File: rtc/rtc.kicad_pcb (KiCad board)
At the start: 2 copper layers, 23.5 x 32.4 mm, 17 parts, among them J1 Conn_02x03_Odd_Even, J2 Conn_01x04, J3 Conn_01x04, J4 Conn_01x04, U1 PCF8563T/5_518, Y1 LFXTAL016178REEL

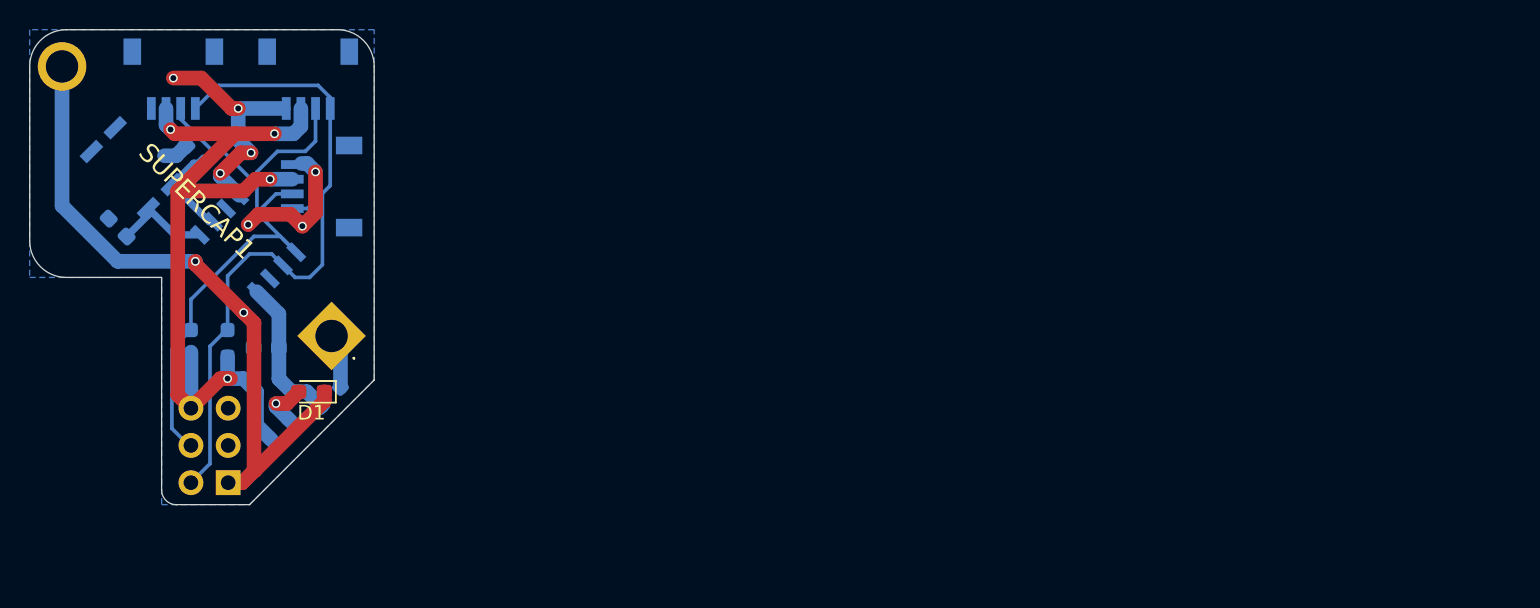
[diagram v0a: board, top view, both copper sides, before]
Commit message: rtc_commit
pushed to git properly
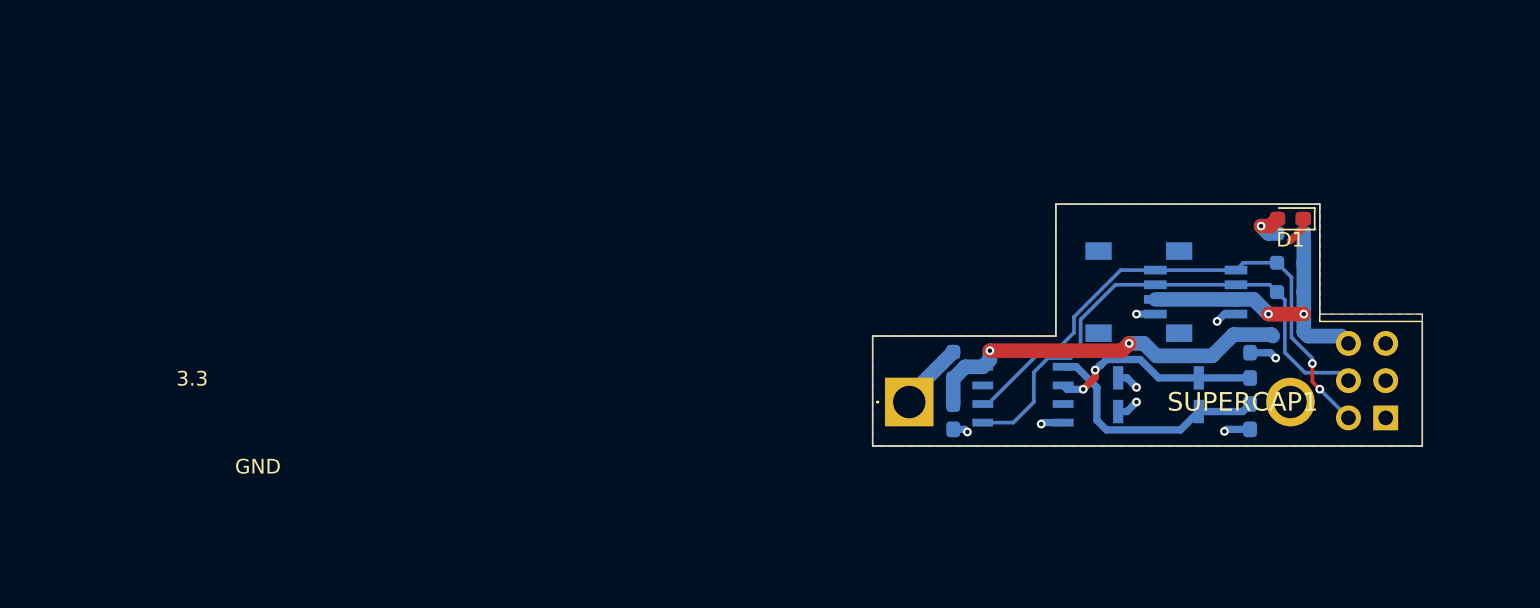
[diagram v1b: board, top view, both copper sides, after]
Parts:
- removed J4: Conn_01x04, pcb_footprints:SM04BSRSSTB
- moved J1 79.1 mm to (233.5, 94.1)
- moved C1 78.3 mm to (224.2, 94.0), turned to -90 degrees
- moved R2 75.1 mm to (227.0, 85.5), turned to 0 degrees
- moved C3 73.4 mm to (224.2, 90.5), turned to 90 degrees
- moved R3 72.7 mm to (227.0, 83.5), turned to 0 degrees
- moved Y1 71.7 mm to (218.0, 92.5), turned to 180 degrees
- moved G*** 70.8 mm to (214.0, 82.5), turned to 180 degrees
- moved R4 70.2 mm to (227.0, 81.5), turned to 180 degrees
- moved D2 69.4 mm to (227.0, 88.5), turned to 0 degrees
- moved D1 67.8 mm to (227.0, 80.5)
- moved J3 60.2 mm to (221.0, 85.5), turned to 90 degrees
- moved J2 57.4 mm to (215.5, 85.5), turned to 90 degrees
- moved U1 53.9 mm to (208.8, 92.5), turned to 180 degrees
- moved C2 47.1 mm to (204.0, 94.0), turned to -90 degrees
- moved R1 42.5 mm to (204.0, 90.5), turned to -90 degrees
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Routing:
- net GND: track 76.1 -> 14.0 mm, vias 9 -> 8
- net +3.3V: track 55.8 -> 20.1 mm, vias 4 -> 2
- net Net-(D2-K): track 10.3 -> 25.9 mm, vias 0 -> 2
- net scl: track 48.3 -> 37.5 mm, vias 0 -> 2
- net Net-(U1-OSCI): track 6.78 -> 16.6 mm
- net sda: track 45.3 -> 36.0 mm
- net Net-(U1-OSCO): track 6.47 -> 14.5 mm, vias 0 -> 2
- net Net-(SUPERCAP1-+): track 3.76 -> 4.66 mm
- net Net-(D1-A): track 3.43 -> 2.63 mm
- added copper zone on F.Cu, net GND
- removed copper zone on B.Cu, net GND
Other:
- board size 23.5 x 32.4 mm -> 37.5 x 16.5 mm
- board text added: "3.3"
- board text added: "GND"
- board text added: "Made by Hailin Chen"
- board text removed: "Designed by A. Ai"

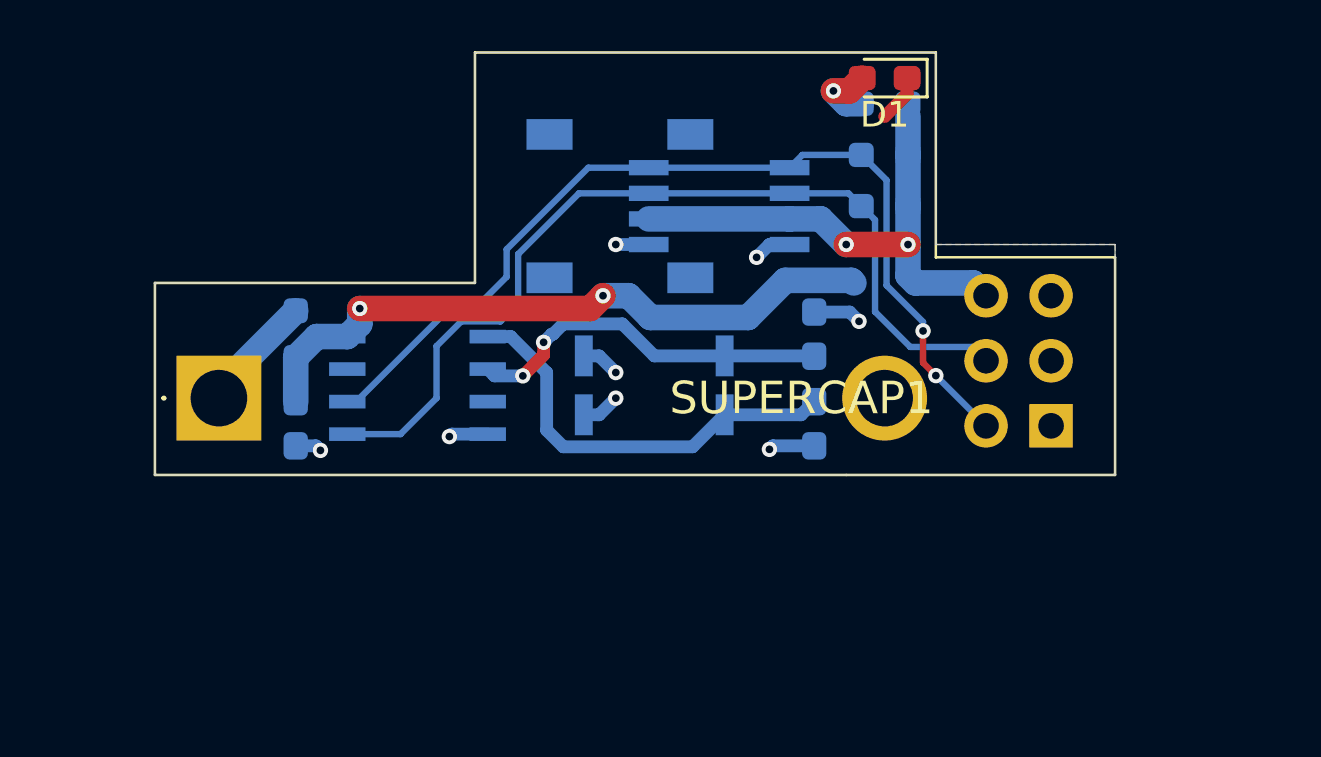
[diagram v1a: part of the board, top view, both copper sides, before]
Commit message: Update rtc.kicad_pcb
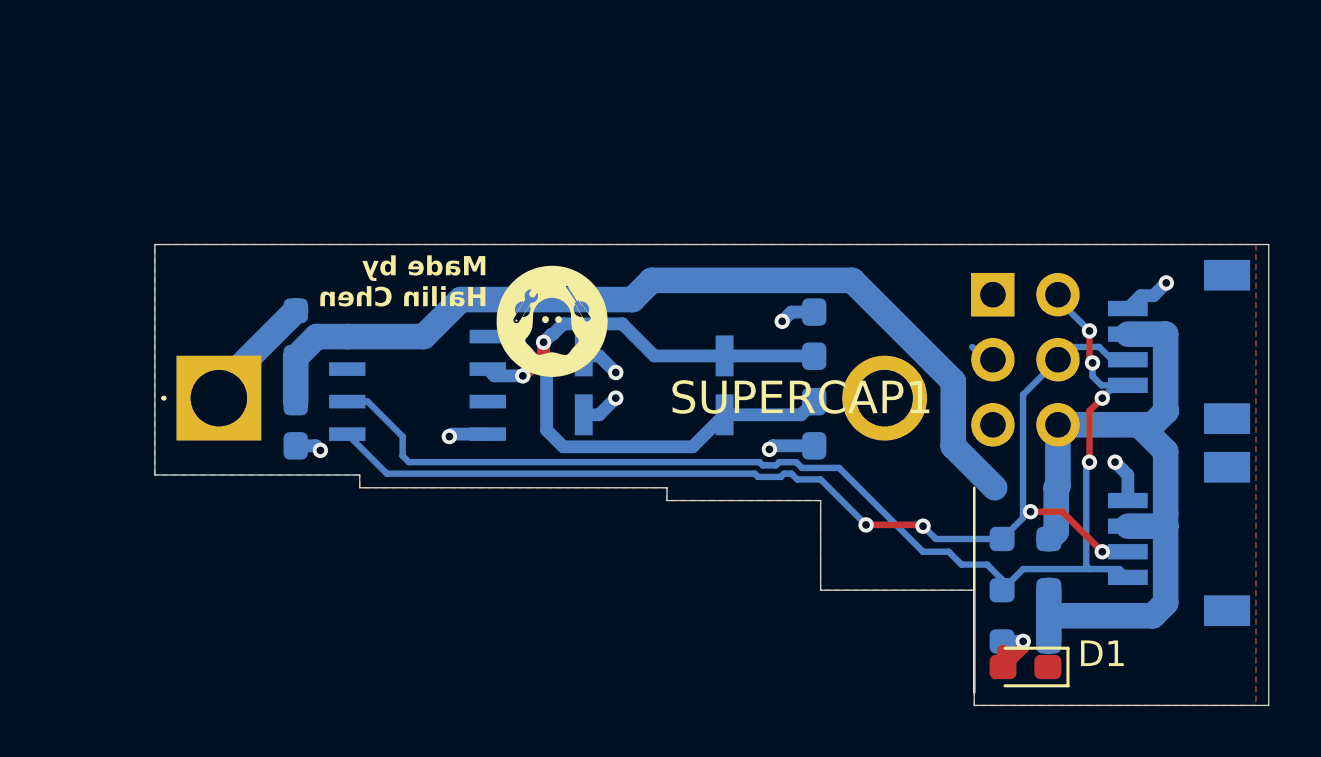
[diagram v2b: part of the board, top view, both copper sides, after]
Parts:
- G***: moved to F.Cu
- moved J2 26.7 mm to (238.8, 98.5), turned to -90 degrees
- moved D1 23.6 mm to (232.5, 103.5)
- moved R4 21.7 mm to (232.5, 102.5)
- moved J3 18.6 mm to (238.8, 91.0), turned to -90 degrees
- moved R3 17.9 mm to (232.5, 100.5)
- moved R2 14.1 mm to (232.5, 98.5)
- moved D2 9.71 mm to (232.5, 96.5)
- moved G*** 7.50 mm to (214.0, 90.0), turned to 0 degrees
- moved J1 5.60 mm to (231.2, 89.0), turned to 180 degrees
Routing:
- net scl: track 37.5 -> 48.5 mm, vias 2 -> 4
- net Net-(D2-K): track 25.9 -> 35.1 mm, vias 2 -> 0
- net +3.3V: track 20.1 -> 29.2 mm, vias 2 -> 0
- net sda: track 36.0 -> 43.2 mm, vias 0 -> 4
- net GND: track 14.0 -> 12.4 mm
- net unconnected-(J1-Pin_3-Pad3): track 0.00 -> 0.76 mm
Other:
- board size 37.5 x 16.5 mm -> 43.5 x 18 mm
